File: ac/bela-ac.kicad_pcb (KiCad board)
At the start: 2 copper layers, 31.8 x 69.9 mm, 30 parts, among them P5 +/-15v, P6 15v_out, P7 belaaudioout, P8 belaaudioin, P9 mod_ac-io, U1 TL074

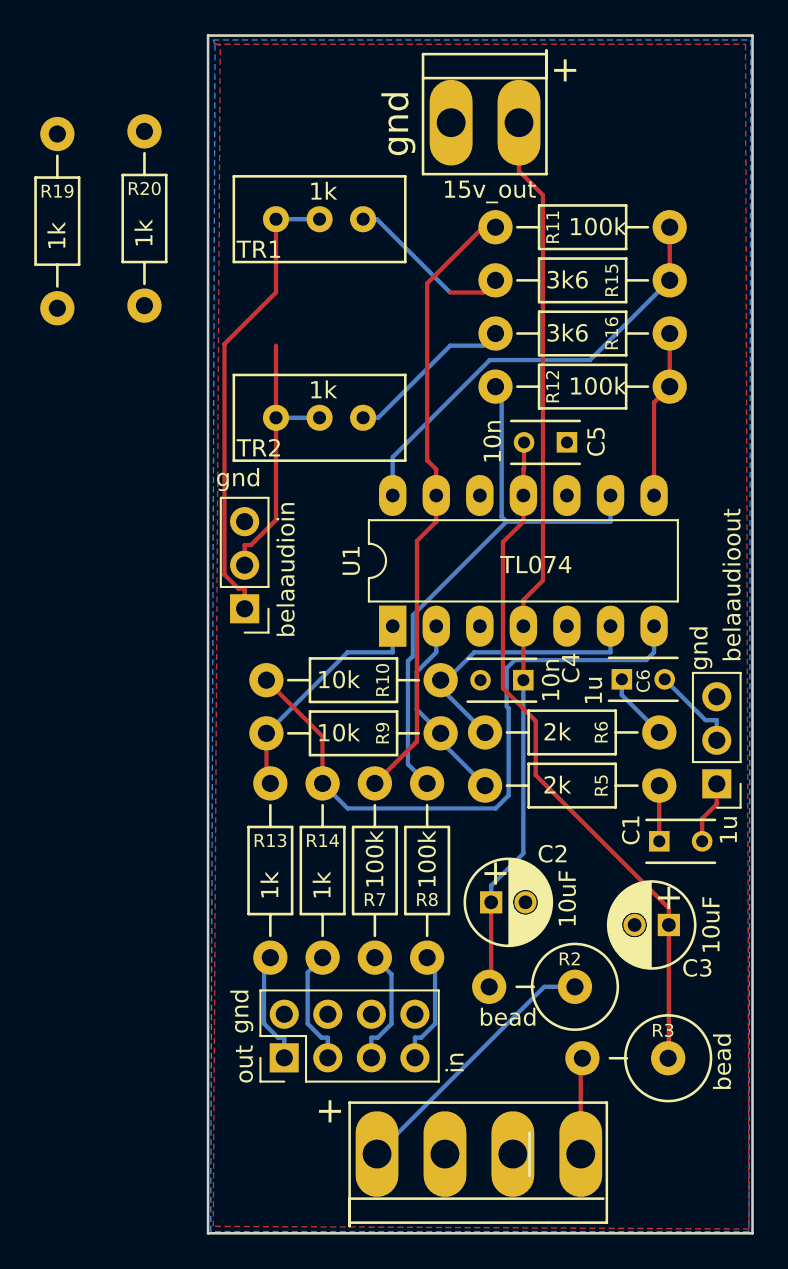
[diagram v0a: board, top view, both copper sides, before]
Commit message: Revert "exchanged bad parts on ac board, though haven't placed yet"
This reverts commit 3185bdf4a96cd7a989377c24179a0fe5be16ab20.
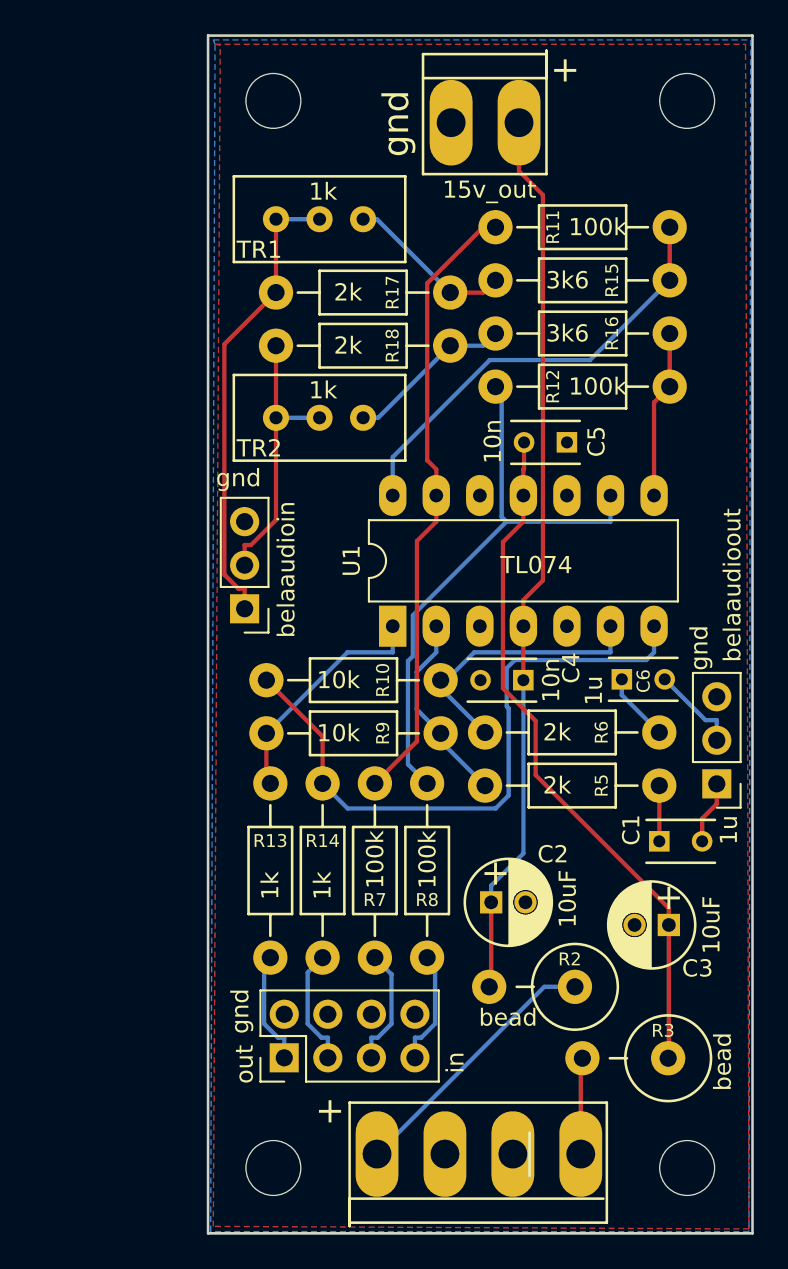
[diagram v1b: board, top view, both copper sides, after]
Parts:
- removed R19, R20: 1k, xnorman:Resistor_Horizontal_RM10mm-xnorman
- added R17: 2k, xnorman:Resistor_Horizontal_RM10mm-xnorman, F.Cu at (29.4, 129.3)
- added R18: 2k, xnorman:Resistor_Horizontal_RM10mm-xnorman, F.Cu at (29.4, 132.4)
- added REF1: MountingHole_3.2mm_M3, Mounting_Holes:MountingHole_3.2mm_M3, F.Cu at (29.2, 118.1)
- added REF2: MountingHole_3.2mm_M3, Mounting_Holes:MountingHole_3.2mm_M3, F.Cu at (53.3, 118.1)
- added REF3: MountingHole_3.2mm_M3, Mounting_Holes:MountingHole_3.2mm_M3, F.Cu at (53.3, 180.3)
- added REF4: MountingHole_3.2mm_M3, Mounting_Holes:MountingHole_3.2mm_M3, F.Cu at (29.2, 180.3)
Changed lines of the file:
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@@
   (general
     (links 59)
-    (no_connects 5)
+    (no_connects 0)
     (area 25.324999 114.224999 57.225001 184.225001)
     (thickness 1.6)
@@
     (tracks 134)
     (zones 0)
-    (modules 30)
+    (modules 34)
     (nets 26)
   )
@@
     )
   )
+  (module xnorman:Resistor_Horizontal_RM10mm-xnorman (layer F.Cu)
+    (at 29.3624 129.286)
+    (descr "Resistor, Axial,  RM 10mm, 1/3W")
+    (tags "Resistor Axial RM 10mm 1/3W")
+    (fp_text reference R17 (at 6.8 0 90) (layer F.SilkS)
+      (effects (font (size 0.75 0.75) (thickness 0.15)))
+    )
+    (fp_text value 2k (at 4.2 0) (layer F.SilkS)
+      (effects (font (size 1 1) (thickness 0.15)))
+    )
+    (fp_line (start -1.25 -1.5) (end 11.4 -1.5) (layer F.CrtYd) (width 0.05))
+    (fp_line (start -1.25 1.5) (end -1.25 -1.5) (layer F.CrtYd) (width 0.05))
+    (fp_line (start 11.4 -1.5) (end 11.4 1.5) (layer F.CrtYd) (width 0.05))
+    (fp_line (start -1.25 1.5) (end 11.4 1.5) (layer F.CrtYd) (width 0.05))
+    (fp_line (start 2.54 -1.27) (end 7.62 -1.27) (layer F.SilkS) (width 0.15))
+    (fp_line (start 7.62 -1.27) (end 7.62 1.27) (layer F.SilkS) (width 0.15))
+    (fp_line (start 7.62 1.27) (end 2.54 1.27) (layer F.SilkS) (width 0.15))
+    (fp_line (start 2.54 1.27) (end 2.54 -1.27) (layer F.SilkS) (width 0.15))
+    (fp_line (start 2.54 0) (end 1.27 0) (layer F.SilkS) (width 0.15))
+    (fp_line (start 7.62 0) (end 8.89 0) (layer F.SilkS) (width 0.15))
+    (pad 1 thru_hole circle (at 0 0) (size 1.99898 1.99898) (drill 1.00076) (layers *.Cu *.SilkS *.Mask)
+      (net 6 belaacin1))
+    (pad 2 thru_hole circle (at 10.16 0) (size 1.99898 1.99898) (drill 1.00076) (layers *.Cu *.SilkS *.Mask)
+      (net 20 "Net-(R15-Pad1)"))
+    (model Resistors_ThroughHole.3dshapes/Resistor_Horizontal_RM10mm.wrl
+      (at (xyz 0.2 0 0))
+      (scale (xyz 0.4 0.4 0.4))
+      (rotate (xyz 0 0 0))
+    )
+  )
+  (module xnorman:Resistor_Horizontal_RM10mm-xnorman (layer F.Cu)
+    (at 29.3624 132.385)
+    (descr "Resistor, Axial,  RM 10mm, 1/3W")
+    (tags "Resistor Axial RM 10mm 1/3W")
+    (fp_text reference R18 (at 6.8 0 90) (layer F.SilkS)
+      (effects (font (size 0.75 0.75) (thickness 0.15)))
+    )
+    (fp_text value 2k (at 4.2 0) (layer F.SilkS)
+      (effects (font (size 1 1) (thickness 0.15)))
+    )
+    (fp_line (start -1.25 -1.5) (end 11.4 -1.5) (layer F.CrtYd) (width 0.05))
+    (fp_line (start -1.25 1.5) (end -1.25 -1.5) (layer F.CrtYd) (width 0.05))
+    (fp_line (start 11.4 -1.5) (end 11.4 1.5) (layer F.CrtYd) (width 0.05))
+    (fp_line (start -1.25 1.5) (end 11.4 1.5) (layer F.CrtYd) (width 0.05))
+    (fp_line (start 2.54 -1.27) (end 7.62 -1.27) (layer F.SilkS) (width 0.15))
+    (fp_line (start 7.62 -1.27) (end 7.62 1.27) (layer F.SilkS) (width 0.15))
+    (fp_line (start 7.62 1.27) (end 2.54 1.27) (layer F.SilkS) (width 0.15))
+    (fp_line (start 2.54 1.27) (end 2.54 -1.27) (layer F.SilkS) (width 0.15))
+    (fp_line (start 2.54 0) (end 1.27 0) (layer F.SilkS) (width 0.15))
+    (fp_line (start 7.62 0) (end 8.89 0) (layer F.SilkS) (width 0.15))
+    (pad 1 thru_hole circle (at 0 0) (size 1.99898 1.99898) (drill 1.00076) (layers *.Cu *.SilkS *.Mask)
+      (net 7 belaacin2))
+    (pad 2 thru_hole circle (at 10.16 0) (size 1.99898 1.99898) (drill 1.00076) (layers *.Cu *.SilkS *.Mask)
+      (net 21 "Net-(R16-Pad1)"))
+    (model Resistors_ThroughHole.3dshapes/Resistor_Horizontal_RM10mm.wrl
+      (at (xyz 0.2 0 0))
+      (scale (xyz 0.4 0.4 0.4))
+      (rotate (xyz 0 0 0))
+    )
+  )
   (module Housings_DIP:DIP-14_W7.62mm_LongPads (layer F.Cu)
     (at 36.1696 148.742 90)
@@
       (net 1 GND))
   )
+  (module Mounting_Holes:MountingHole_3.2mm_M3 (layer F.Cu)
+    (at 29.21 118.11)
+    (descr "Mounting Hole 3.2mm, no annular, M3")
+    (tags "mounting hole 3.2mm no annular m3")
+    (fp_text reference REF1 (at 0 -4.2) (layer F.SilkS) hide
+      (effects (font (size 1 1) (thickness 0.15)))
+    )
+    (fp_text value MountingHole_3.2mm_M3 (at 0 4.2) (layer F.Fab) hide
+      (effects (font (size 1 1) (thickness 0.15)))
+    )
+    (fp_circle (center 0 0) (end 3.2 0) (layer Cmts.User) (width 0.15))
+    (fp_circle (center 0 0) (end 3.45 0) (layer F.CrtYd) (width 0.05))
+    (pad 1 np_thru_hole circle (at 0 0) (size 3.2 3.2) (drill 3.2) (layers *.Cu *.Mask))
+  )
+  (module Mounting_Holes:MountingHole_3.2mm_M3 (layer F.Cu)
+    (at 53.34 118.11)
+    (descr "Mounting Hole 3.2mm, no annular, M3")
+    (tags "mounting hole 3.2mm no annular m3")
+    (fp_text reference REF2 (at 0 -4.2) (layer F.SilkS) hide
+      (effects (font (size 1 1) (thickness 0.15)))
+    )
+    (fp_text value MountingHole_3.2mm_M3 (at 0 4.2) (layer F.Fab) hide
+      (effects (font (size 1 1) (thickness 0.15)))
+    )
+    (fp_circle (center 0 0) (end 3.2 0) (layer Cmts.User) (width 0.15))
+    (fp_circle (center 0 0) (end 3.45 0) (layer F.CrtYd) (width 0.05))
+    (pad 1 np_thru_hole circle (at 0 0) (size 3.2 3.2) (drill 3.2) (layers *.Cu *.Mask))
+  )
+  (module Mounting_Holes:MountingHole_3.2mm_M3 (layer F.Cu)
+    (at 29.21 180.34)
+    (descr "Mounting Hole 3.2mm, no annular, M3")
+    (tags "mounting hole 3.2mm no annular m3")
+    (fp_text reference REF4 (at 0 -4.2) (layer F.SilkS) hide
+      (effects (font (size 1 1) (thickness 0.15)))
+    )
+    (fp_text value MountingHole_3.2mm_M3 (at 0 4.2) (layer F.Fab) hide
+      (effects (font (size 1 1) (thickness 0.15)))
+    )
+    (fp_circle (center 0 0) (end 3.2 0) (layer Cmts.User) (width 0.15))
+    (fp_circle (center 0 0) (end 3.45 0) (layer F.CrtYd) (width 0.05))
+    (pad 1 np_thru_hole circle (at 0 0) (size 3.2 3.2) (drill 3.2) (layers *.Cu *.Mask))
+  )
+  (module Mounting_Holes:MountingHole_3.2mm_M3 (layer F.Cu)
+    (at 53.34 180.34)
+    (descr "Mounting Hole 3.2mm, no annular, M3")
+    (tags "mounting hole 3.2mm no annular m3")
+    (fp_text reference REF3 (at 0 -4.2) (layer F.SilkS) hide
+      (effects (font (size 1 1) (thickness 0.15)))
+    )
+    (fp_text value MountingHole_3.2mm_M3 (at 0 4.2) (layer F.Fab) hide
+      (effects (font (size 1 1) (thickness 0.15)))
+    )
+    (fp_circle (center 0 0) (end 3.2 0) (layer Cmts.User) (width 0.15))
+    (fp_circle (center 0 0) (end 3.45 0) (layer F.CrtYd) (width 0.05))
+    (pad 1 np_thru_hole circle (at 0 0) (size 3.2 3.2) (drill 3.2) (layers *.Cu *.Mask))
+  )
   (module Capacitors_ThroughHole:C_Rect_L4_W2.5_P2.5 (layer F.Cu)
     (at 51.7144 161.29)
@@
       (net 21 "Net-(R16-Pad1)"))
   )
-  (module xnorman:Resistor_Horizontal_RM10mm-xnorman (layer F.Cu)
-    (at 16.6116 130.2004 90)
-    (descr "Resistor, Axial,  RM 10mm, 1/3W")
-    (tags "Resistor Axial RM 10mm 1/3W")
-    (fp_text reference R19 (at 6.8 0 180) (layer F.SilkS)
-      (effects (font (size 0.75 0.75) (thickness 0.15)))
-    )
-    (fp_text value 1k (at 4.2 0 90) (layer F.SilkS)
-      (effects (font (size 1 1) (thickness 0.15)))
-    )
-    (fp_line (start -1.25 -1.5) (end 11.4 -1.5) (layer F.CrtYd) (width 0.05))
-    (fp_line (start -1.25 1.5) (end -1.25 -1.5) (layer F.CrtYd) (width 0.05))
-    (fp_line (start 11.4 -1.5) (end 11.4 1.5) (layer F.CrtYd) (width 0.05))
-    (fp_line (start -1.25 1.5) (end 11.4 1.5) (layer F.CrtYd) (width 0.05))
-    (fp_line (start 2.54 -1.27) (end 7.62 -1.27) (layer F.SilkS) (width 0.15))
-    (fp_line (start 7.62 -1.27) (end 7.62 1.27) (layer F.SilkS) (width 0.15))
-    (fp_line (start 7.62 1.27) (end 2.54 1.27) (layer F.SilkS) (width 0.15))
-    (fp_line (start 2.54 1.27) (end 2.54 -1.27) (layer F.SilkS) (width 0.15))
-    (fp_line (start 2.54 0) (end 1.27 0) (layer F.SilkS) (width 0.15))
-    (fp_line (start 7.62 0) (end 8.89 0) (layer F.SilkS) (width 0.15))
-    (pad 1 thru_hole circle (at 0 0 90) (size 1.99898 1.99898) (drill 1.00076) (layers *.Cu *.SilkS *.Mask)
-      (net 1 GND))
-    (pad 2 thru_hole circle (at 10.16 0 90) (size 1.99898 1.99898) (drill 1.00076) (layers *.Cu *.SilkS *.Mask)
-      (net 6 belaacin1))
-    (model Resistors_ThroughHole.3dshapes/Resistor_Horizontal_RM10mm.wrl
-      (at (xyz 0.2 0 0))
-      (scale (xyz 0.4 0.4 0.4))
-      (rotate (xyz 0 0 0))
-    )
-  )
-  (module xnorman:Resistor_Horizontal_RM10mm-xnorman (layer F.Cu)
-    (at 21.6916 130.048 90)
-    (descr "Resistor, Axial,  RM 10mm, 1/3W")
-    (tags "Resistor Axial RM 10mm 1/3W")
-    (fp_text reference R20 (at 6.8 0 180) (layer F.SilkS)
-      (effects (font (size 0.75 0.75) (thickness 0.15)))
-    )
-    (fp_text value 1k (at 4.2 0 90) (layer F.SilkS)
-      (effects (font (size 1 1) (thickness 0.15)))
-    )
-    (fp_line (start -1.25 -1.5) (end 11.4 -1.5) (layer F.CrtYd) (width 0.05))
-    (fp_line (start -1.25 1.5) (end -1.25 -1.5) (layer F.CrtYd) (width 0.05))
-    (fp_line (start 11.4 -1.5) (end 11.4 1.5) (layer F.CrtYd) (width 0.05))
-    (fp_line (start -1.25 1.5) (end 11.4 1.5) (layer F.CrtYd) (width 0.05))
-    (fp_line (start 2.54 -1.27) (end 7.62 -1.27) (layer F.SilkS) (width 0.15))
-    (fp_line (start 7.62 -1.27) (end 7.62 1.27) (layer F.SilkS) (width 0.15))
-    (fp_line (start 7.62 1.27) (end 2.54 1.27) (layer F.SilkS) (width 0.15))
-    (fp_line (start 2.54 1.27) (end 2.54 -1.27) (layer F.SilkS) (width 0.15))
-    (fp_line (start 2.54 0) (end 1.27 0) (layer F.SilkS) (width 0.15))
-    (fp_line (start 7.62 0) (end 8.89 0) (layer F.SilkS) (width 0.15))
-    (pad 1 thru_hole circle (at 0 0 90) (size 1.99898 1.99898) (drill 1.00076) (layers *.Cu *.SilkS *.Mask)
-      (net 1 GND))
-    (pad 2 thru_hole circle (at 10.16 0 90) (size 1.99898 1.99898) (drill 1.00076) (layers *.Cu *.SilkS *.Mask)
-      (net 7 belaacin2))
-    (model Resistors_ThroughHole.3dshapes/Resistor_Horizontal_RM10mm.wrl
-      (at (xyz 0.2 0 0))
-      (scale (xyz 0.4 0.4 0.4))
-      (rotate (xyz 0 0 0))
-    )
-  )
   (gr_text http://x37v.info (at 40.9956 144.8308) (layer B.SilkS)
